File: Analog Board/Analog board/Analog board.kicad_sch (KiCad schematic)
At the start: 84 parts, among them J1 a, J2 b, J3 Conn_01x04, U1 LM324, U2 LM324, U3 LM339

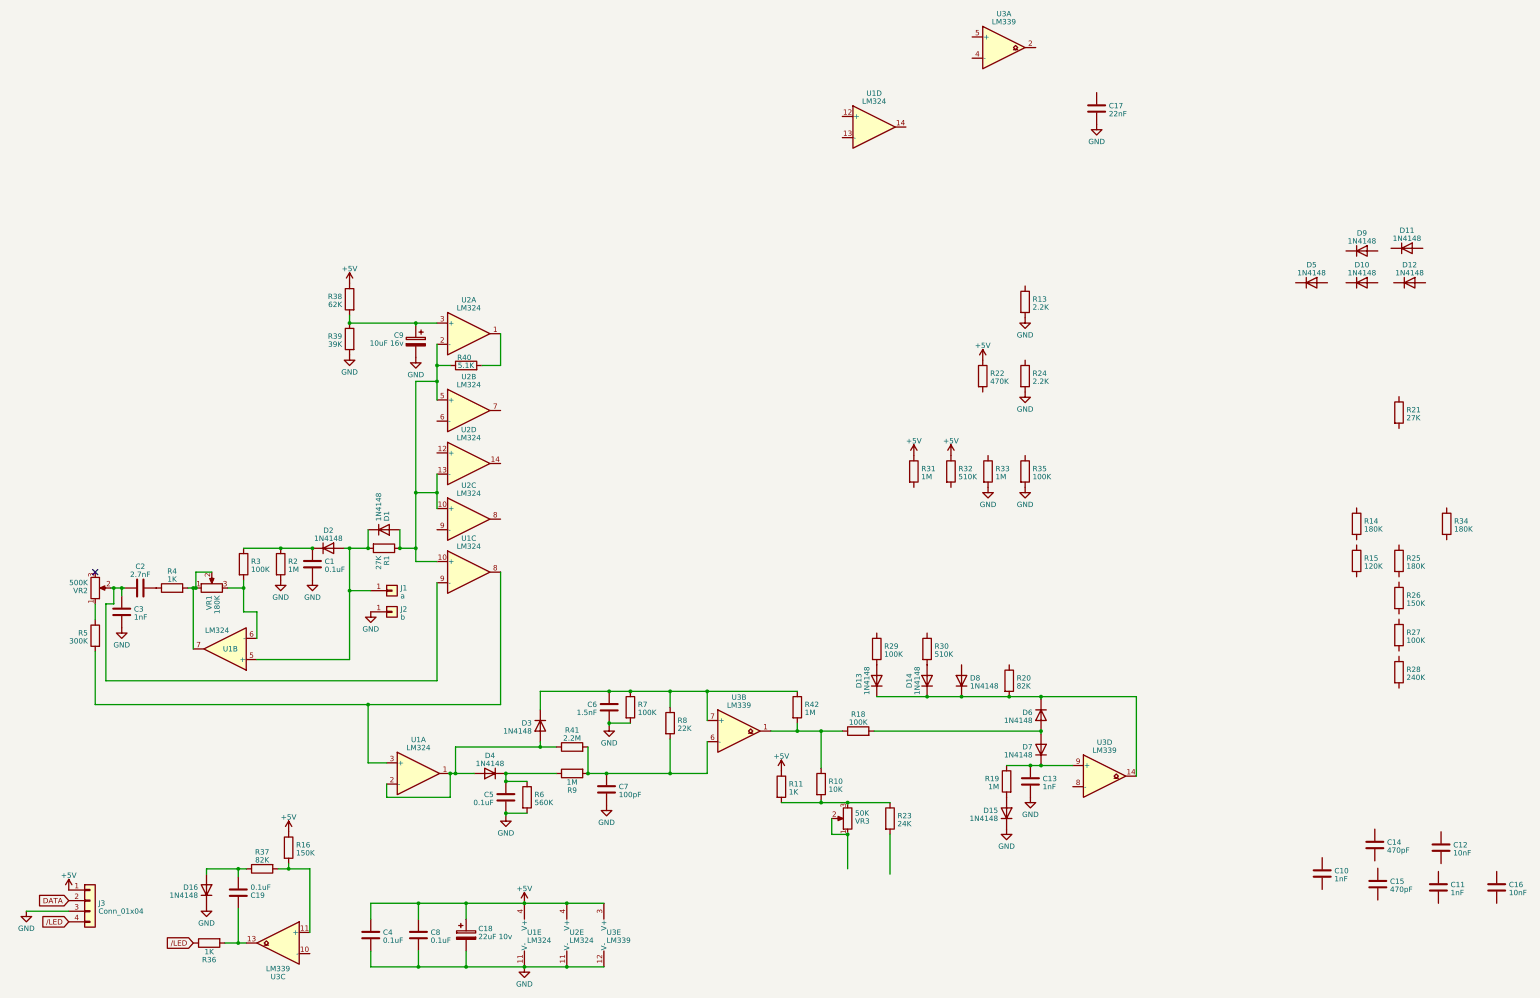
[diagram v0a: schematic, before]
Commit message: finished messy layout
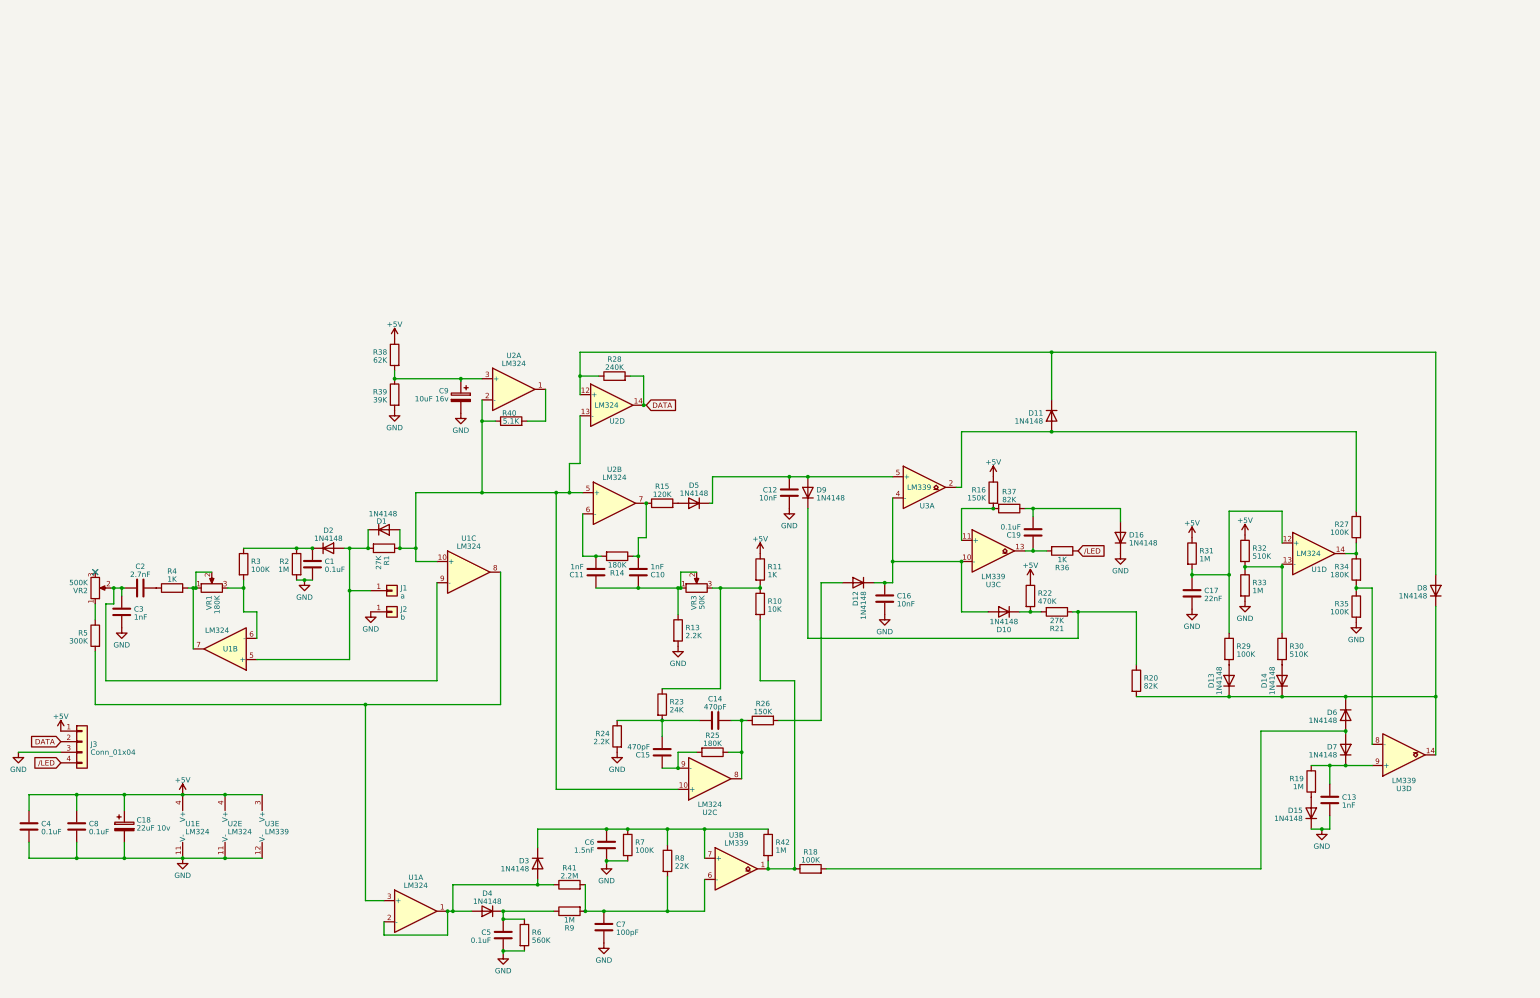
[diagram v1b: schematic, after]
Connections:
- net DATA: now also R28.2, U2.14
- net GND: now also C12.2, C16.2
- net at R34.1: now also R27.2, U1.14
- net at R34.2: now also R35.1, U3.8 (-)
- net at U2.6 (-): now also C11.2, R14.2
- net at U2.7: now also C10.2, R14.1, R15.1
- net at R30.1: now also R32.2, R33.1, U1.13 (-)
- net at R15.2: now also D5.2 (A)
- net at VR3.1, VR3.2: now also C10.1, C11.1, R13.1
- net at R11.2, R23.1, VR3.3: now also R10.1; no longer R10.2
- net at D10.1 (K): now also R21.2, R22.2
- net at D10.2 (A): now also C16.1, D12.1 (K), U3.10 (-), U3.4 (-)
- net at D11.1 (K): now also D8.2 (A), R28.1, U2.12 (+)
- net at D11.2 (A): now also R27.1, U3.2
- net at D5.1 (K): now also C12.1, D9.2 (A), U3.5 (+)
- net at C14.1: now also C15.2, R23.2, R24.1
- net at C14.2: now also R25.1, R26.1, U2.8
- net at D12.2 (A): now also R26.2
- net at R18.1, R42.2, U3.1: now also R10.2; no longer R10.1
- net at R29.1: now also C17.1, R31.2, U1.12 (+)
- net at U2.9 (-): now also C15.1, R25.2
- net at D9.1 (K): now also R20.1, R21.1
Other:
- moved on the sheet: C10, C11, C12, C13, C14, C15, C16, C17, C18, C19, C4, C5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

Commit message: better layout
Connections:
- net at C3.1, U1.9 (-), VR2.2: now also C2.2; no longer C2.1
- net at R4.1: now also C2.1; no longer C2.2
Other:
- note added: "VR1 is fixed value at 180K"
- moved on the sheet: C1, C10, C11, C12, C13, C14, C15, C16, C17, C18, C19, C2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

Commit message: finished rough layout
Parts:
- C1, C10, C11, C12, C13, C14, C15, C16, C17, C19, C2, C3, C4, C5, C6, C7, C8: footprint (none) -> Capacitor_THT:C_Disc_D4.7mm_W2.5mm_P5.00mm
- C18, C9: footprint (none) -> Capacitor_THT:CP_Radial_D5.0mm_P2.50mm
- D1, D10, D11, D12, D13, D14, D15, D16, D2, D3, D4, D5, D6, D7, D8, D9: footprint Diode_THT:D_DO-35_SOD27_P7.62mm_Horizontal -> Diode_THT:D_DO-35_SOD27_P10.16mm_Horizontal
- J1, J2: footprint (none) -> Connector_PinHeader_2.54mm:PinHeader_1x01_P2.54mm_Vertical
- J3: footprint (none) -> Connector_PinHeader_2.54mm:PinHeader_2x02_P2.54mm_Vertical
- R1, R10, R11, R13, R14, R15, R16, R18, R19, R2, R20, R21, R22, R23, R24, R25, R26, R27, R28, R29, R3, R30, R31, R32, R33, R34, R35, R36, R37, R38, R39, R4, R40, R41, R42, R5, R6, R7, R8, R9: footprint (none) -> Resistor_THT:R_Axial_DIN0207_L6.3mm_D2.5mm_P10.16mm_Horizontal
- U1, U2, U3: footprint (none) -> Package_DIP:DIP-14_W7.62mm
- VR1, VR2, VR3: footprint (none) -> Potentiometer_THT:Potentiometer_ACP_CA9-V10_Vertical
